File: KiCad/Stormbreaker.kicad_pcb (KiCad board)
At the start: 4 copper layers, 50.2 x 21 mm, 50 parts, among them J1 Micro_SD_Card_Det2, J2 USB_C_Receptacle_USB2.0_14P, J3 PROG, J4 FAN, J5 I2C, Q1 PMOS, Q2 NMOS, SW1 SW_Push, U1 BQ25895RTW, U3 ATtiny1616-M, U4 HUSB238A

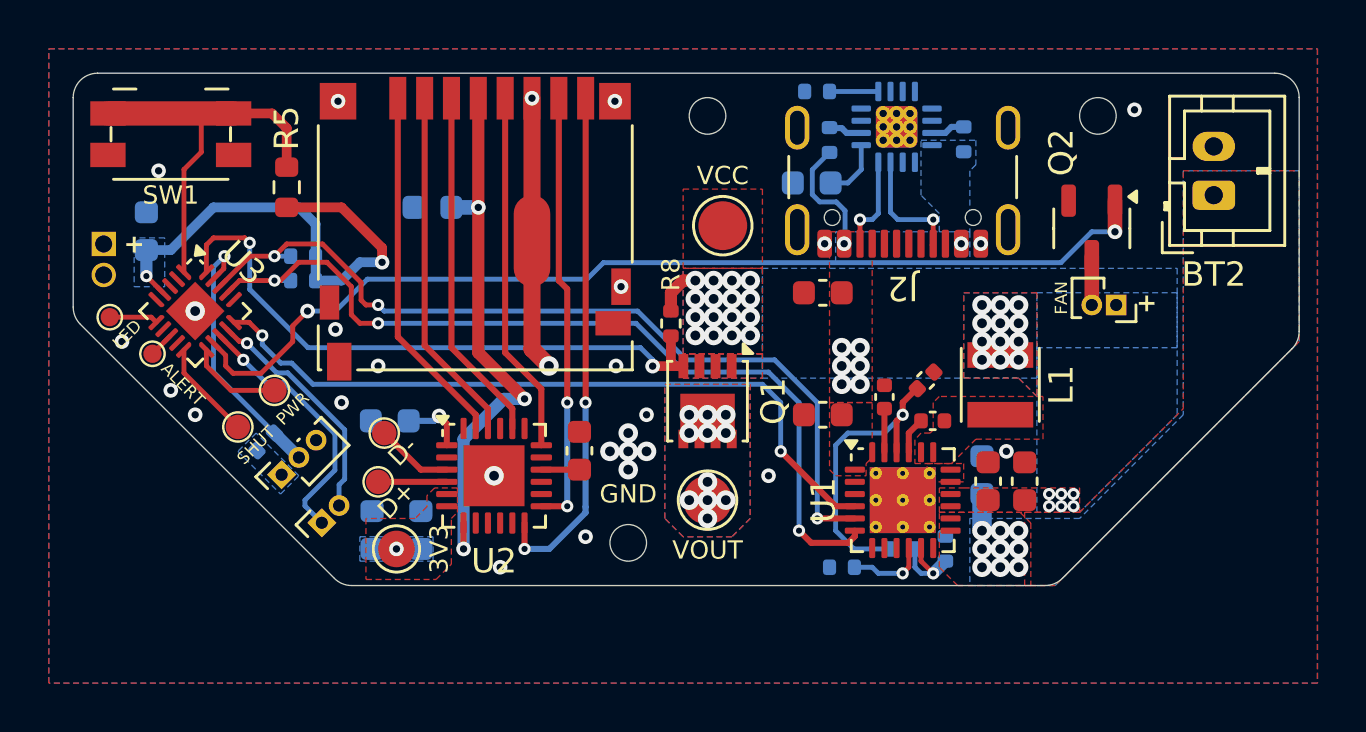
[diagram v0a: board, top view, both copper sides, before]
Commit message: Misc improvements
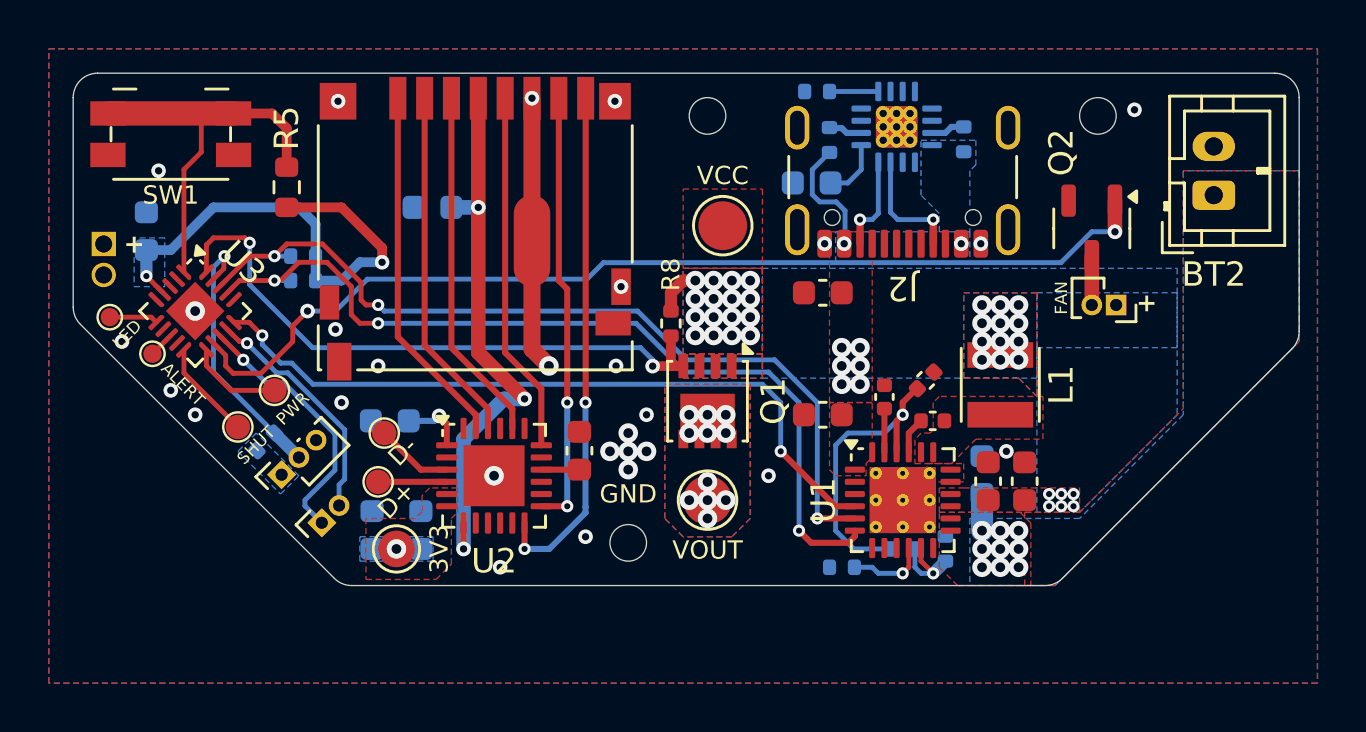
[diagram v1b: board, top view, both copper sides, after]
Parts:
- C1: value 1uF -> 10uF
